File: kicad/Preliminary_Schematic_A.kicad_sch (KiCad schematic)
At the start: 13 parts, among them J1 Battery Connection, J2 Load Cell System, M1 Motor_Servo, Q1 DMN2075U-7, U1 VL53L4CDV0DH/1

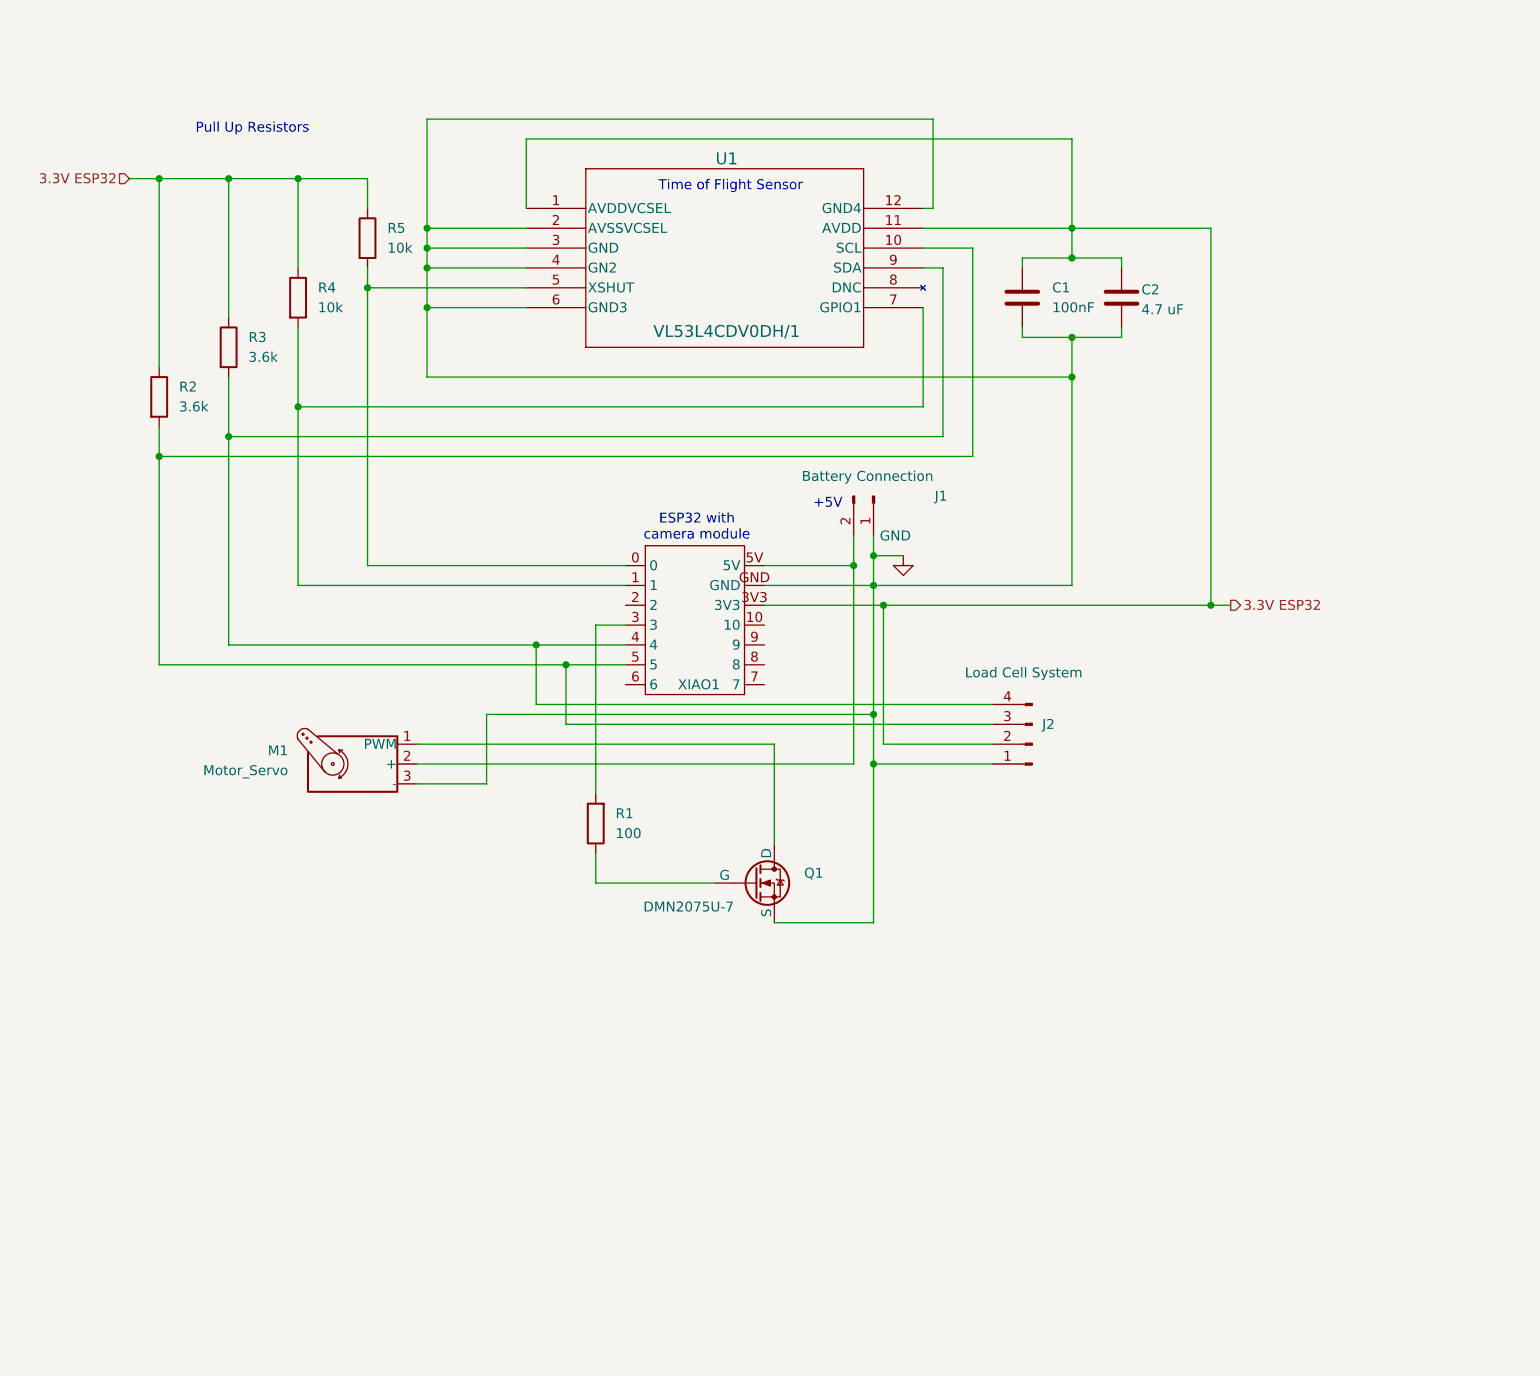
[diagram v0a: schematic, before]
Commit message: Add files via upload
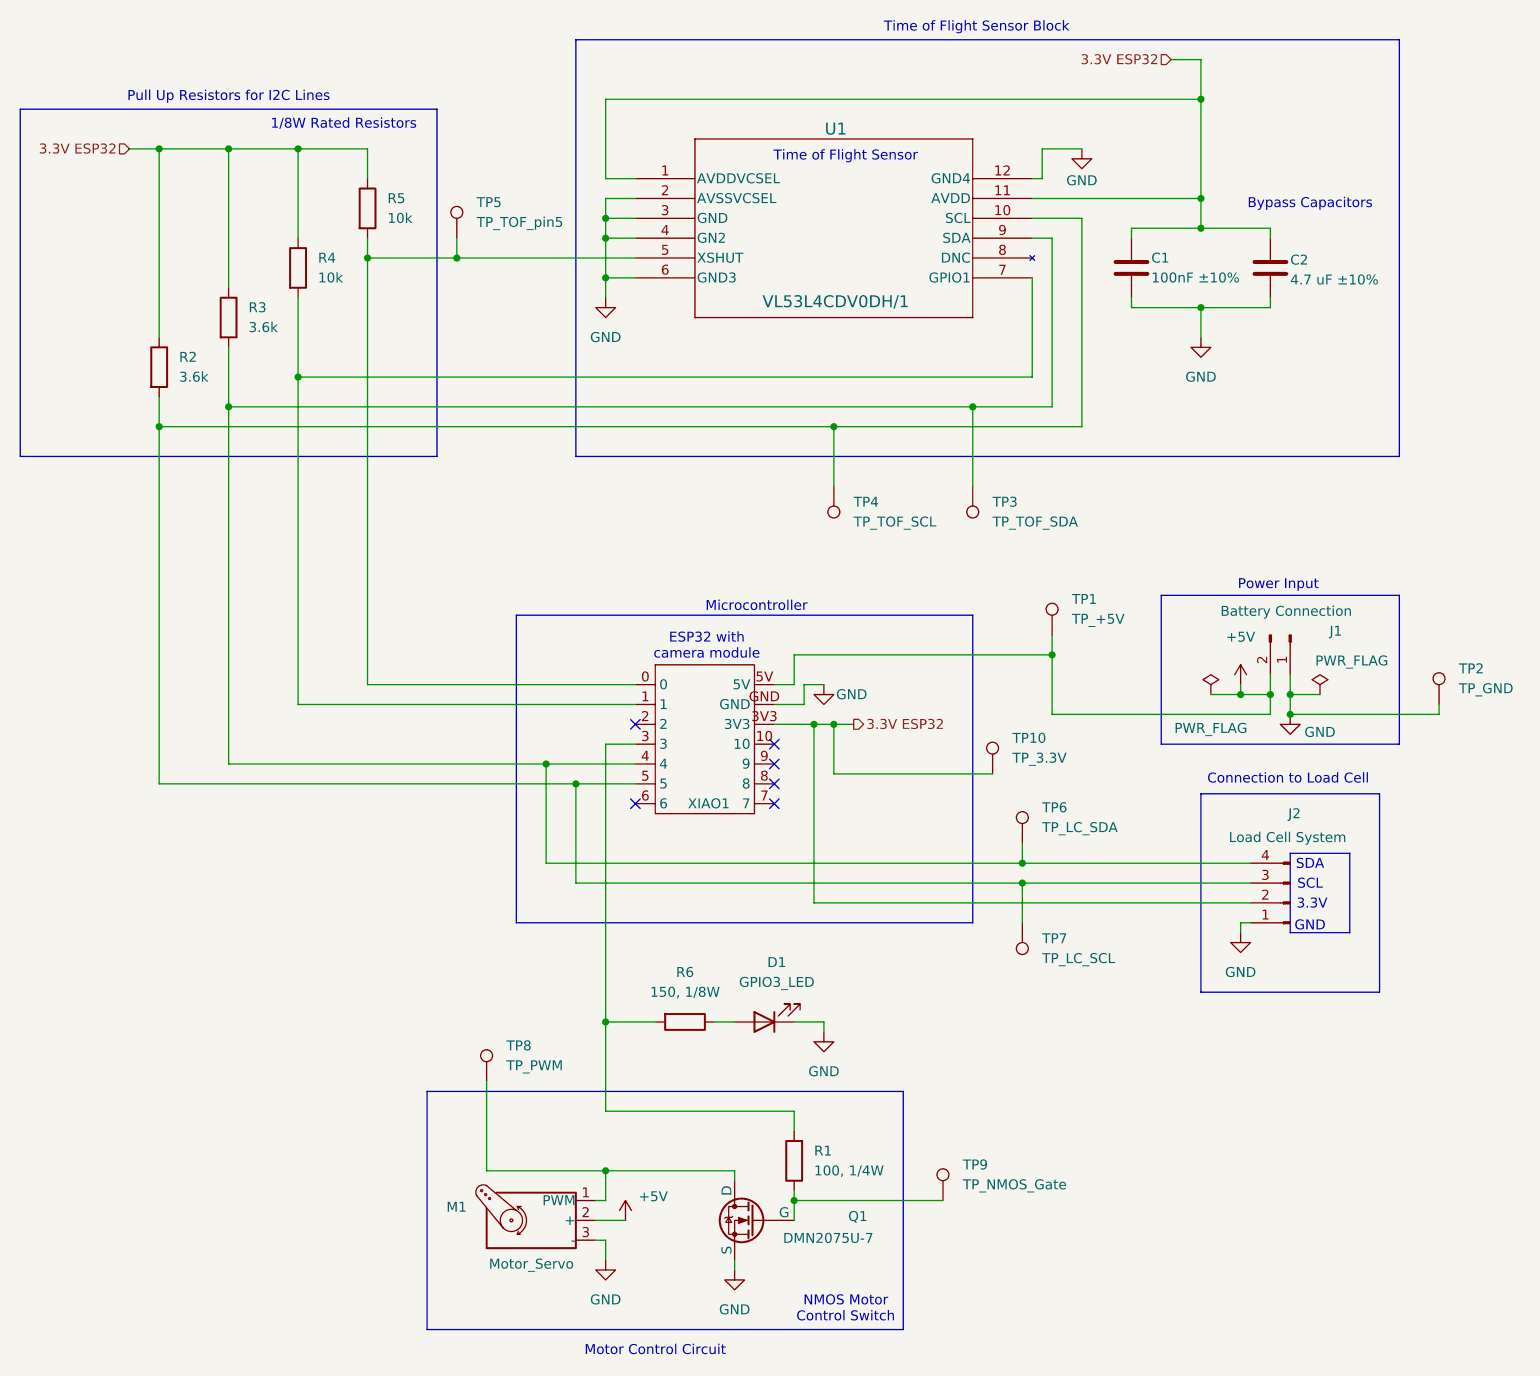
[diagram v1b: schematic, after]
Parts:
- added D1: GPIO3_LED, Connector_PinHeader_2.54mm:PinHeader_1x02_P2.54mm_Vertical, symbol Device:LED
- added R6: 150, 1/8W, Resistor_SMD:R_0805_2012Metric_Pad1.20x1.40mm_HandSolder, symbol Device:R
- added TP1: TP_+5V, TestPoint:TestPoint_THTPad_D2.0mm_Drill1.0mm, symbol Connector:TestPoint
- added TP10: TP_3.3V, TestPoint:TestPoint_THTPad_D2.0mm_Drill1.0mm, symbol Connector:TestPoint
- added TP2: TP_GND, TestPoint:TestPoint_THTPad_D2.0mm_Drill1.0mm, symbol Connector:TestPoint
- added TP3: TP_TOF_SDA, TestPoint:TestPoint_THTPad_D2.0mm_Drill1.0mm, symbol Connector:TestPoint
- added TP4: TP_TOF_SCL, TestPoint:TestPoint_THTPad_D2.0mm_Drill1.0mm, symbol Connector:TestPoint
- added TP5: TP_TOF_pin5, TestPoint:TestPoint_THTPad_D2.0mm_Drill1.0mm, symbol Connector:TestPoint
- added TP6: TP_LC_SDA, TestPoint:TestPoint_THTPad_D2.0mm_Drill1.0mm, symbol Connector:TestPoint
- added TP7: TP_LC_SCL, TestPoint:TestPoint_THTPad_D2.0mm_Drill1.0mm, symbol Connector:TestPoint
- added TP8: TP_PWM, TestPoint:TestPoint_THTPad_D2.0mm_Drill1.0mm, symbol Connector:TestPoint
- added TP9: TP_NMOS_Gate, TestPoint:TestPoint_THTPad_D2.0mm_Drill1.0mm, symbol Connector:TestPoint
- C1: value 100nF -> 100nF ±10%
- C2: value 4.7 uF -> 4.7 uF ±10%
- R1: value 100 -> 100, 1/4W
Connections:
- net 3.3V ESP32: now also TP10.1
- net GND: now also D1.1 (K), TP2.1
- net +5V: now reaches J1.2 (Pin_2), M1.2 (+), XIAO1.5V
- net +5V: now also TP1.1
- net at J2.3 (Pin_3), R2.2, U1.10 (SCL)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: now also TP4.1, TP7.1
- net at M1.1 (PWM), Q1.1 (D): now also TP8.1
- net at Q1.2 (G), R1.1: now also TP9.1
- net at R5.2, U1.5 (XSHUT), XIAO1.0: now also TP5.1
- net at R1.2, XIAO1.3: now also R6.2
- net at J2.4 (Pin_4), R3.2, U1.9 (SDA)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: now also TP3.1, TP6.1
- new net: D1.2 (A), R6.1
- no-connect marks 0 -> 6
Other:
- note added: "1/8W Rated Resistors"
- note added: "3.3V"
- note added: "Bypass Capacitors"
- note added: "Connection to Load Cell"
- note added: "GND"
- note added: "Microcontroller"
- note added: "Motor Control Circuit"
- note added: "NMOS Motor Control Switch"
- note added: "Power Input"
- note added: "Pull Up Resistors for I2C Lines"
- note added: "SCL"
- note added: "SDA"
- note added: "Time of Flight Sensor Block"
- note removed: "+5V"
- note removed: "Pull Up Resistors"
- moved on the sheet: C1, C2, J1, J2, M1, Q1, R1, R2, R3, R4, R5, U1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
